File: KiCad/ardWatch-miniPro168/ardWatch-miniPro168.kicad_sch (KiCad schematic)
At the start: 6 parts, among them J1 2-pin_power_input_header, U1 Arduino_Mini_Pro, U3 ST7735_1.8"_TFT_128x160, U4 DS3231_RTC_module

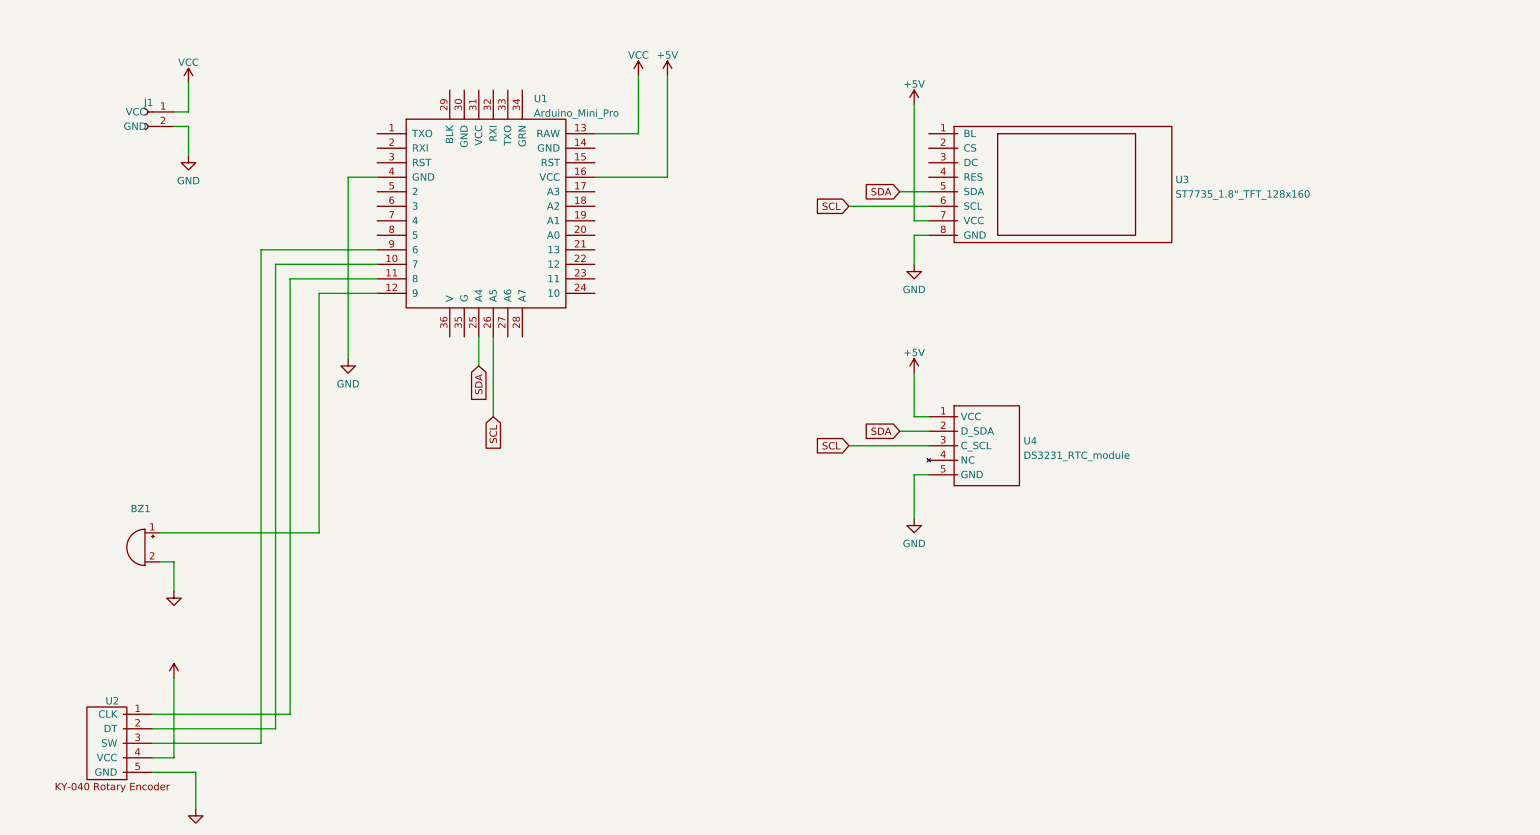
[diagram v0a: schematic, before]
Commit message: renames, code
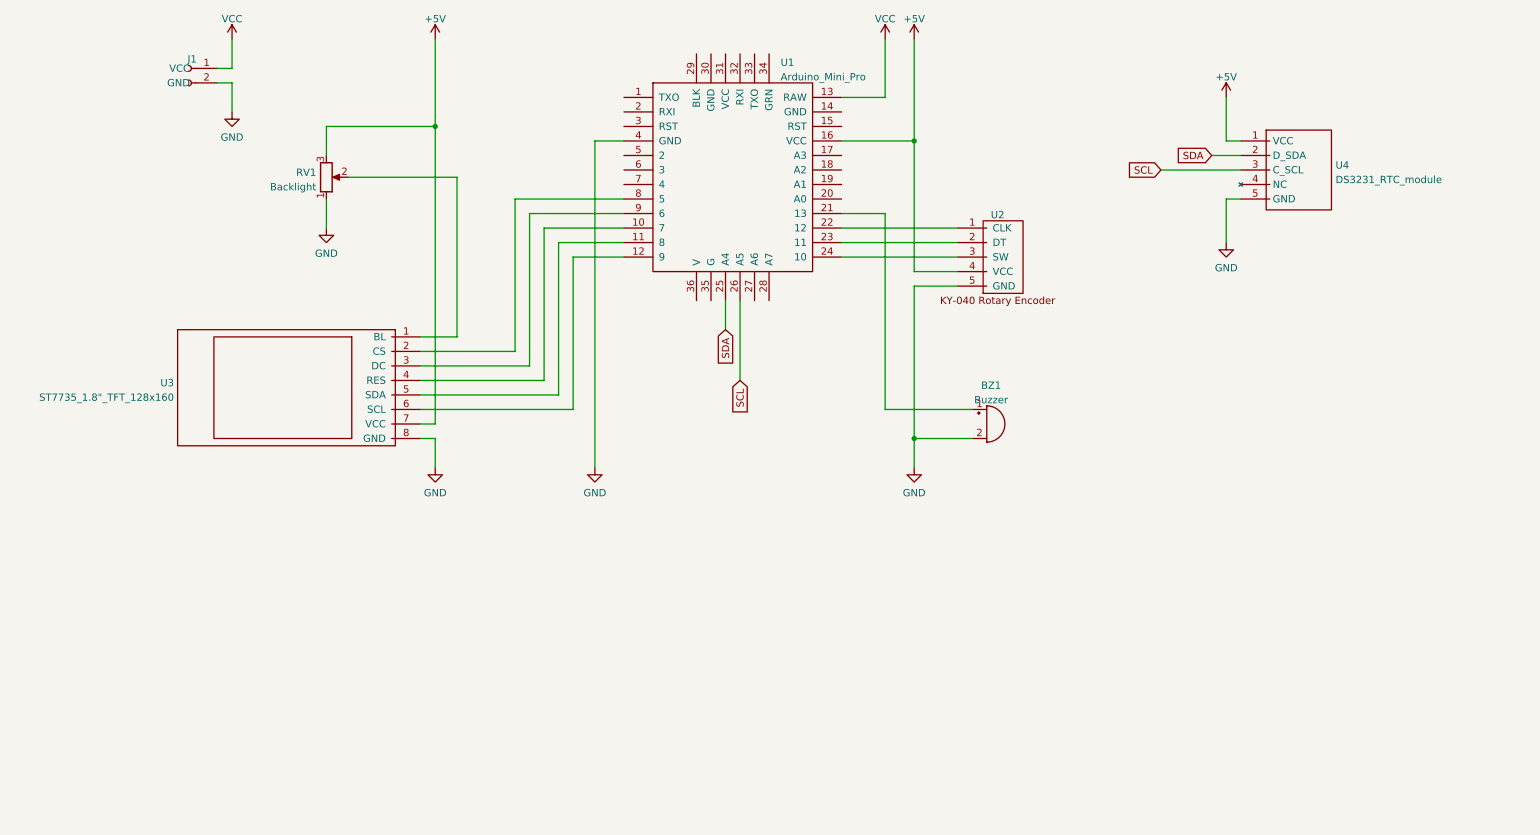
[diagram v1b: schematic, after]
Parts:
- added RV1: Backlight, My_Misc:Potentiometer_Bourns_3339P_Vertical_large, symbol Device:R_Potentiometer
- BZ1: value (none) -> Buzzer; footprint (none) -> My_Misc:Buzzer_TDK_PS1240P02BT_D12.2mm_H6.5mm_large
- U2: value (none) -> KY-040_Rotary_Encoder; footprint (none) -> My_Parts:KY-040_rotary_encoder module_w_header_large
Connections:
- net +5V: now also RV1.3
- net GND: now also RV1.1
- net SCL: no longer U3.6 (SCL)
- net SDA: no longer U3.5 (SDA)
- net at U1.10 (7): now also U3.4 (RES); no longer U2.2 (DT)
- net at U1.11 (8): now also U3.5 (SDA); no longer U2.1 (CLK)
- net at U1.12 (9): now also U3.6 (SCL); no longer BZ1.1 (-)
- net at U1.21 (13): now also BZ1.1 (-)
- net at U1.22 (12): now also U2.1 (CLK)
- net at U1.23 (11): now also U2.2 (DT)
- net at U1.24 (10): now also U2.3 (SW)
- net at U1.8 (5): now also U3.2 (CS)
- net at U1.9 (6): now also U3.3 (DC); no longer U2.3 (SW)
- net at U3.1 (BL): now also RV1.2
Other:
- moved on the sheet: BZ1, J1, U1, U2, U3, U4

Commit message: kicad v8
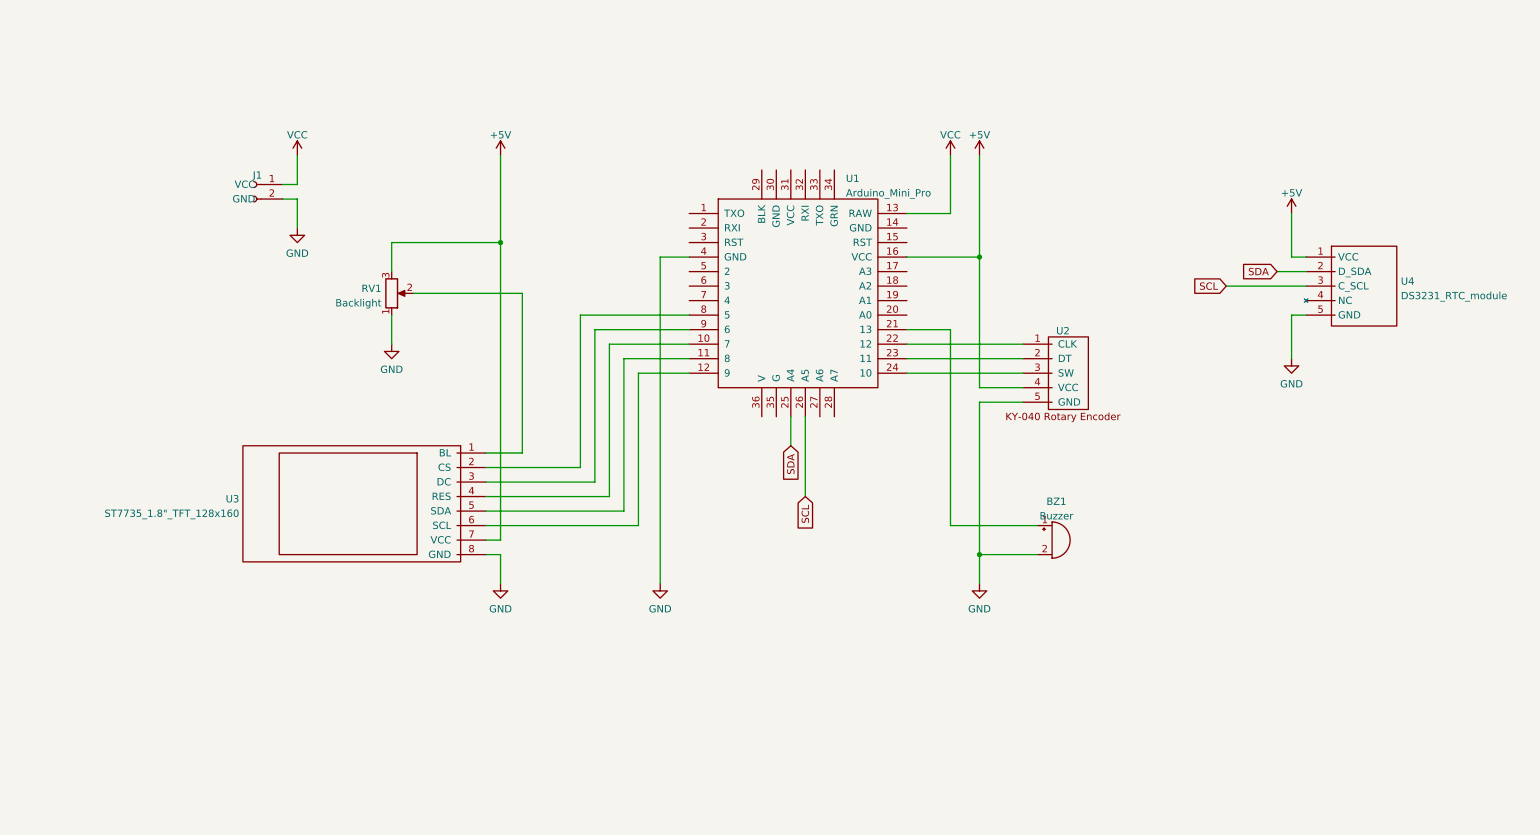
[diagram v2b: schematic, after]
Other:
- moved on the sheet: BZ1, J1, RV1, U1, U2, U3, U4
